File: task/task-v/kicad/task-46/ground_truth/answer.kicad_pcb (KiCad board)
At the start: 2 copper layers, 80 x 80 mm, 8 parts

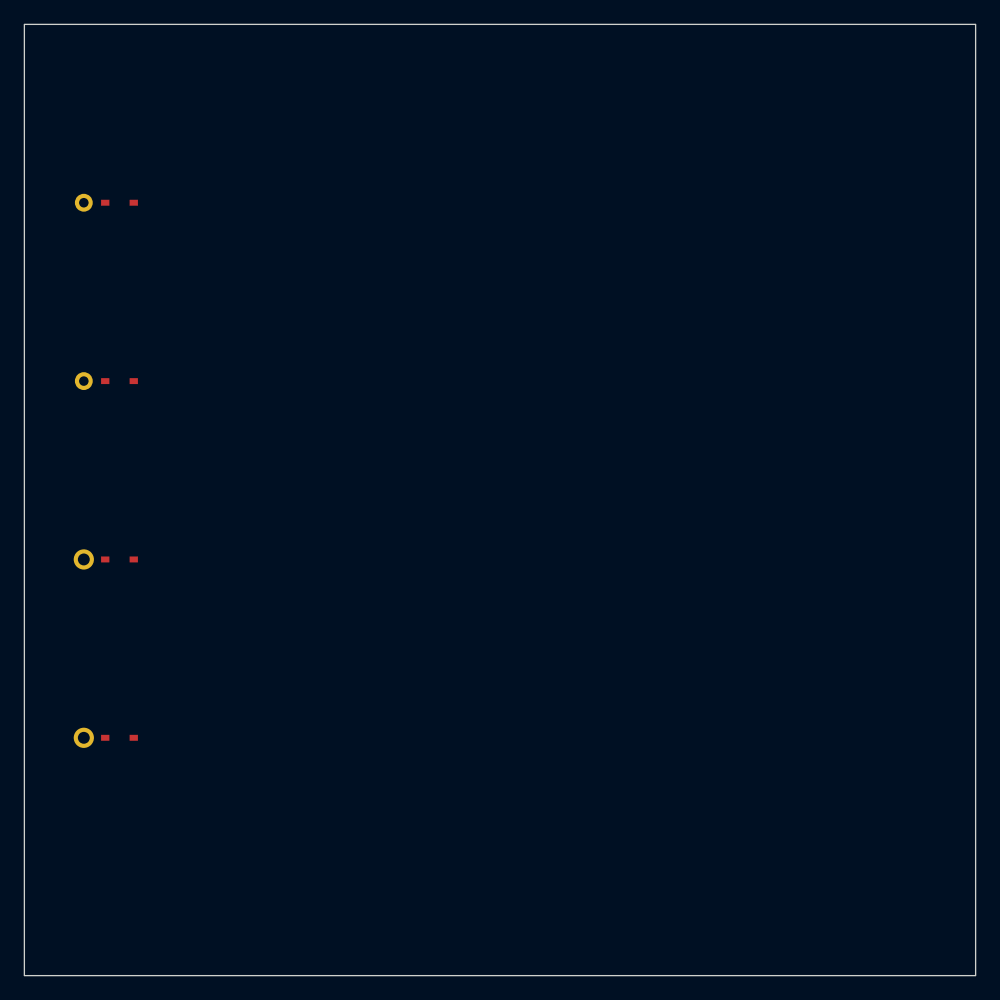
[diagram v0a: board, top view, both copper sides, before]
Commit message: Refine engineering task metadata and instructions
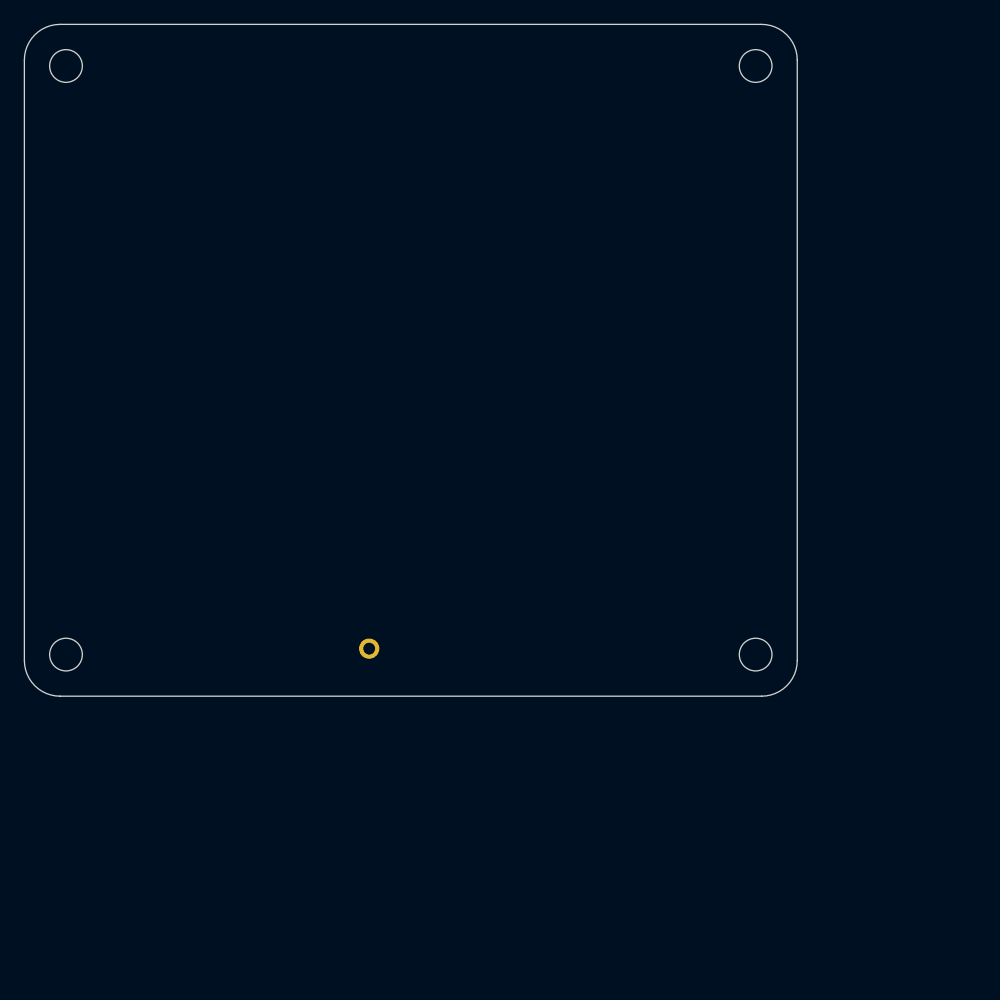
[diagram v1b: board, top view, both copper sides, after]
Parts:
- removed the ? at (5.00, 15.0)
- removed the ? at (5.00, 30.0)
- removed the ? at (5.00, 45.0)
- removed the ? at (5.00, 60.0)
- removed the ? at (8.00, 15.0)
- removed the ? at (8.00, 30.0)
- removed the ? at (8.00, 45.0)
- removed the ? at (8.00, 60.0)
- added ?: , MountingHole:MountingHole_2.75mm_M2.5, F.Cu at (3.50, 3.50)
- added ?: , MountingHole:MountingHole_2.75mm_M2.5, F.Cu at (61.5, 3.50)
- added ?: , MountingHole:MountingHole_2.75mm_M2.5, F.Cu at (3.50, 53.0)
- added ?: , MountingHole:MountingHole_2.75mm_M2.5, F.Cu at (61.5, 53.0)
- added ?: , Connector_PinHeader_2.54mm:PinHeader_2x20_P2.54mm_Vertical, F.Cu at (29.0, 52.5)
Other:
- board size 80 x 80 mm -> 65 x 56.5 mm
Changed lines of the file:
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@@
   )
   (net 0 "")
-  (net 1 "USB_DP")
-  (net 2 "USB_DM")
-  (net 3 "SIG_TX")
-  (net 4 "SIG_RX")
-  (net 5 "GND")
-  ; Connectors unchanged
-  (footprint "Connector_USB:USB_A_Molex_67643_Vertical" (layer "F.Cu") (at 5 15)
-    (reference "J1") (value "USB-A")
-    (pad "1" thru_hole circle (at 0 0) (size 1.5 1.5) (drill 0.8)
-      (layers "F.Cu" "B.Cu" "F.Mask" "B.Mask") (net 1 "USB_DP"))
+  (net 1 "VCC")
+  (net 2 "GND")
+  ; HAT+ board outline: 65x56.5mm with R=3mm rounded corners
+  ; Straight edges
+  (gr_line (start 3 0) (end 62 0) (layer "Edge.Cuts") (width 0.1))
+  (gr_line (start 65 3) (end 65 53.5) (layer "Edge.Cuts") (width 0.1))
+  (gr_line (start 62 56.5) (end 3 56.5) (layer "Edge.Cuts") (width 0.1))
+  (gr_line (start 0 53.5) (end 0 3) (layer "Edge.Cuts") (width 0.1))
+  ; Rounded corners (gr_arc: start, mid, end)
+  ; Bottom-left corner: center(3,3), R=3, arc from (0,3) through (0.879,0.879) to (3,0)
+  (gr_arc (start 0 3) (mid 0.879 0.879) (end 3 0) (layer "Edge.Cuts") (width 0.1))
+  ; Bottom-right corner: center(62,3), R=3, arc from (62,0) through (64.121,0.879) to (65,3)
+  (gr_arc (start 62 0) (mid 64.121 0.879) (end 65 3) (layer "Edge.Cuts") (width 0.1))
+  ; Top-right corner: center(62,53.5), R=3, arc from (65,53.5) through (64.121,55.621) to (62,56.5)
+  (gr_arc (start 65 53.5) (mid 64.121 55.621) (end 62 56.5) (layer "Edge.Cuts") (width 0.1))
+  ; Top-left corner: center(3,53.5), R=3, arc from (3,56.5) through (0.879,55.621) to (0,53.5)
+  (gr_arc (start 3 56.5) (mid 0.879 55.621) (end 0 53.5) (layer "Edge.Cuts") (width 0.1))
+  ; 4 M2.5 mounting holes at HAT+ spec positions
+  (footprint "MountingHole:MountingHole_2.75mm_M2.5" (layer "F.Cu") (at 3.5 3.5)
+    (reference "H1") (value "MountingHole")
+    (pad "" np_thru_hole circle (at 0 0) (size 2.75 2.75) (drill 2.75)
+      (layers "F.Cu" "B.Cu" "F.Mask" "B.Mask"))
   )
-  (footprint "Connector_USB:USB_A_Molex_67643_Vertical" (layer "F.Cu") (at 5 30)
-    (reference "J2") (value "USB-A")
-    (pad "1" thru_hole circle (at 0 0) (size 1.5 1.5) (drill 0.8)
-      (layers "F.Cu" "B.Cu" "F.Mask" "B.Mask") (net 2 "USB_DM"))
+  (footprint "MountingHole:MountingHole_2.75mm_M2.5" (layer "F.Cu") (at 61.5 3.5)
+    (reference "H2") (value "MountingHole")
+    (pad "" np_thru_hole circle (at 0 0) (size 2.75 2.75) (drill 2.75)
+      (layers "F.Cu" "B.Cu" "F.Mask" "B.Mask"))
   )
-  (footprint "Connector_PinHeader_2.54mm:PinHeader_1x04_P2.54mm_Vertical" (layer "F.Cu") (at 5 45)
-    (reference "J3") (value "CONN-4P")
+  (footprint "MountingHole:MountingHole_2.75mm_M2.5" (layer "F.Cu") (at 3.5 53)
+    (reference "H3") (value "MountingHole")
+    (pad "" np_thru_hole circle (at 0 0) (size 2.75 2.75) (drill 2.75)
+      (layers "F.Cu" "B.Cu" "F.Mask" "B.Mask"))
+  )
+  (footprint "MountingHole:MountingHole_2.75mm_M2.5" (layer "F.Cu") (at 61.5 53)
+    (reference "H4") (value "MountingHole")
+    (pad "" np_thru_hole circle (at 0 0) (size 2.75 2.75) (drill 2.75)
+      (layers "F.Cu" "B.Cu" "F.Mask" "B.Mask"))
+  )
+  ; 2x20 GPIO header repositioned to HAT+ spec position (29.0, 52.5)
+  (footprint "Connector_PinHeader_2.54mm:PinHeader_2x20_P2.54mm_Vertical" (layer "F.Cu") (at 29.0 52.5)
+    (reference "J1") (value "GPIO_HEADER")
     (pad "1" thru_hole circle (at 0 0) (size 1.7 1.7) (drill 1.0)
-      (layers "F.Cu" "B.Cu" "F.Mask" "B.Mask") (net 3 "SIG_TX"))
+      (layers "F.Cu" "B.Cu" "F.Mask" "B.Mask") (net 1 "VCC"))
   )
-  (footprint "Connector_PinHeader_2.54mm:PinHeader_1x04_P2.54mm_Vertical" (layer "F.Cu") (at 5 60)
-    (reference "J4") (value "CONN-4P")
-    (pad "1" thru_hole circle (at 0 0) (size 1.7 1.7) (drill 1.0)
-      (layers "F.Cu" "B.Cu" "F.Mask" "B.Mask") (net 4 "SIG_RX"))
-  )
-  ; ESD arrays moved close to connectors (within 5mm of connector pads)
-  ; D1 moved to (8, 15): D1.pad1 at (8-1.2, 15)=(6.8,15), J1.pad at (5,15), dist=1.8mm <= 5mm
-  (footprint "Package_TO_SOT_SMD:SOT-363_SC-70-6" (layer "F.Cu") (at 8 15)
-    (reference "D1") (value "PRTR5V0U2X")
-    (pad "1" smd rect (at -1.2 0) (size 0.7 0.5)
-      (layers "F.Cu" "F.Paste" "F.Mask") (net 1 "USB_DP"))
-    (pad "6" smd rect (at 1.2 0) (size 0.7 0.5)
-      (layers "F.Cu" "F.Paste" "F.Mask") (net 5 "GND"))
-  )
-  ; D2 moved to (8, 30): D2.pad1 at (6.8,30), J2.pad at (5,30), dist=1.8mm <= 5mm
-  (footprint "Package_TO_SOT_SMD:SOT-363_SC-70-6" (layer "F.Cu") (at 8 30)
-    (reference "D2") (value "PRTR5V0U2X")
-    (pad "1" smd rect (at -1.2 0) (size 0.7 0.5)
-      (layers "F.Cu" "F.Paste" "F.Mask") (net 2 "USB_DM"))
-    (pad "6" smd rect (at 1.2 0) (size 0.7 0.5)
-      (layers "F.Cu" "F.Paste" "F.Mask") (net 5 "GND"))
-  )
-  ; D3 moved to (8, 45): D3.pad1 at (6.8,45), J3.pad at (5,45), dist=1.8mm <= 5mm
-  (footprint "Package_TO_SOT_SMD:SOT-363_SC-70-6" (layer "F.Cu") (at 8 45)
-    (reference "D3") (value "PRTR5V0U2X")
-    (pad "1" smd rect (at -1.2 0) (size 0.7 0.5)
-      (layers "F.Cu" "F.Paste" "F.Mask") (net 3 "SIG_TX"))
-    (pad "6" smd rect (at 1.2 0) (size 0.7 0.5)
-      (layers "F.Cu" "F.Paste" "F.Mask") (net 5 "GND"))
-  )
-  ; D4 moved to (8, 60): D4.pad1 at (6.8,60), J4.pad at (5,60), dist=1.8mm <= 5mm
-  (footprint "Package_TO_SOT_SMD:SOT-363_SC-70-6" (layer "F.Cu") (at 8 60)
-    (reference "D4") (value "PRTR5V0U2X")
-    (pad "1" smd rect (at -1.2 0) (size 0.7 0.5)
-      (layers "F.Cu" "F.Paste" "F.Mask") (net 4 "SIG_RX"))
-    (pad "6" smd rect (at 1.2 0) (size 0.7 0.5)
-      (layers "F.Cu" "F.Paste" "F.Mask") (net 5 "GND"))
-  )
-  (gr_rect (start 0 0) (end 80 80) (layer "Edge.Cuts") (width 0.1))
 )
